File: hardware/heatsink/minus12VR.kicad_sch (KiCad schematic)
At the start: 3 parts

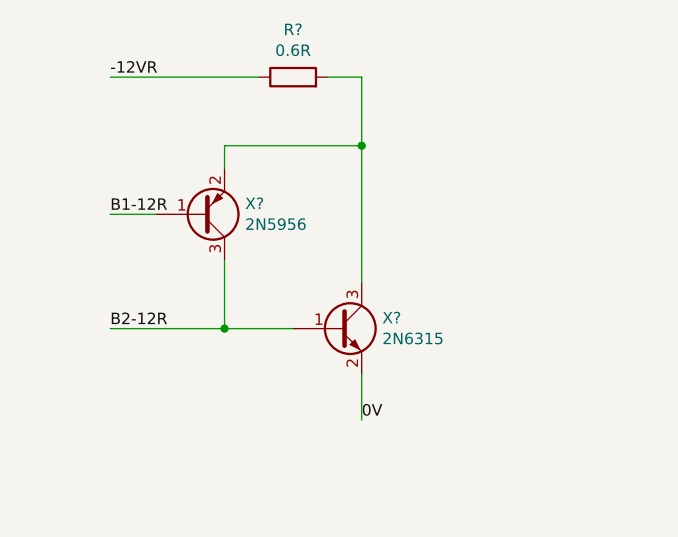
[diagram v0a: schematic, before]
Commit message: small update in schematic
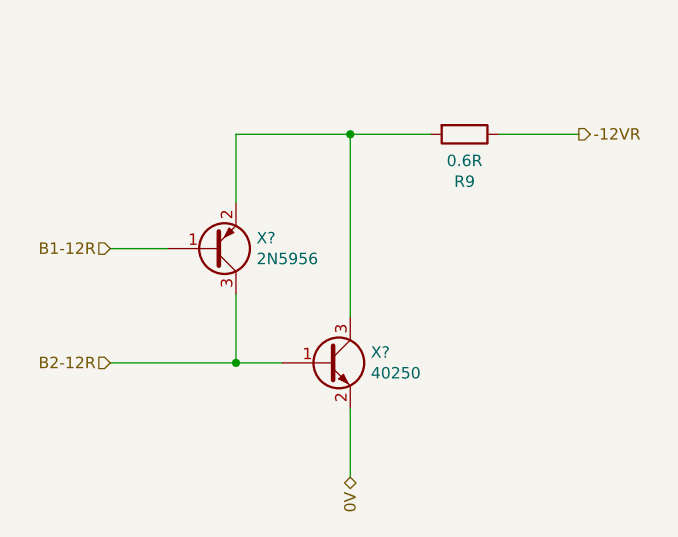
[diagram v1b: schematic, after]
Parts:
- X?: value 2N6315 -> 40250
- gave numbers to parts that had none: 1
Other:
- moved on the sheet: R9, X?
